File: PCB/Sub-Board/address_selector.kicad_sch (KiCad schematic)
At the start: 10 parts, among them SW1 SW_DIP_x07

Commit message: Sub Board PCB: PCB Layout (wip)
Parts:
- R10, R11, R12, R13, R5, R6, R7, R8, R9: footprint Resistor_SMD:R_0603_1608Metric -> Resistor_SMD:R_0402_1005Metric
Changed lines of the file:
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@@
 			)
 		)
-		(property "Footprint" "Resistor_SMD:R_0603_1608Metric"
+		(property "Footprint" "Resistor_SMD:R_0402_1005Metric"
 			(at 87.122 83.82 90)
 			(effects
@@
 			)
 		)
-		(property "Footprint" "Resistor_SMD:R_0603_1608Metric"
+		(property "Footprint" "Resistor_SMD:R_0402_1005Metric"
 			(at 109.982 83.82 90)
 			(effects
@@
 			)
 		)
-		(property "Footprint" "Resistor_SMD:R_0603_1608Metric"
+		(property "Footprint" "Resistor_SMD:R_0402_1005Metric"
 			(at 79.502 83.82 90)
 			(effects
@@
 			)
 		)
-		(property "Footprint" "Resistor_SMD:R_0603_1608Metric"
+		(property "Footprint" "Resistor_SMD:R_0402_1005Metric"
 			(at 117.602 55.88 90)
 			(effects
@@
 			)
 		)
-		(property "Footprint" "Resistor_SMD:R_0603_1608Metric"
+		(property "Footprint" "Resistor_SMD:R_0402_1005Metric"
 			(at 94.742 83.82 90)
 			(effects
@@
 			)
 		)
-		(property "Footprint" "Resistor_SMD:R_0603_1608Metric"
+		(property "Footprint" "Resistor_SMD:R_0402_1005Metric"
 			(at 64.262 83.82 90)
 			(effects
@@
 			)
 		)
-		(property "Footprint" "Resistor_SMD:R_0603_1608Metric"
+		(property "Footprint" "Resistor_SMD:R_0402_1005Metric"
 			(at 39.37 71.628 90)
 			(effects
@@
 			)
 		)
-		(property "Footprint" "Resistor_SMD:R_0603_1608Metric"
+		(property "Footprint" "Resistor_SMD:R_0402_1005Metric"
 			(at 102.362 83.82 90)
 			(effects
@@
 			)
 		)
-		(property "Footprint" "Resistor_SMD:R_0603_1608Metric"
+		(property "Footprint" "Resistor_SMD:R_0402_1005Metric"
 			(at 71.882 83.82 90)
 			(effects

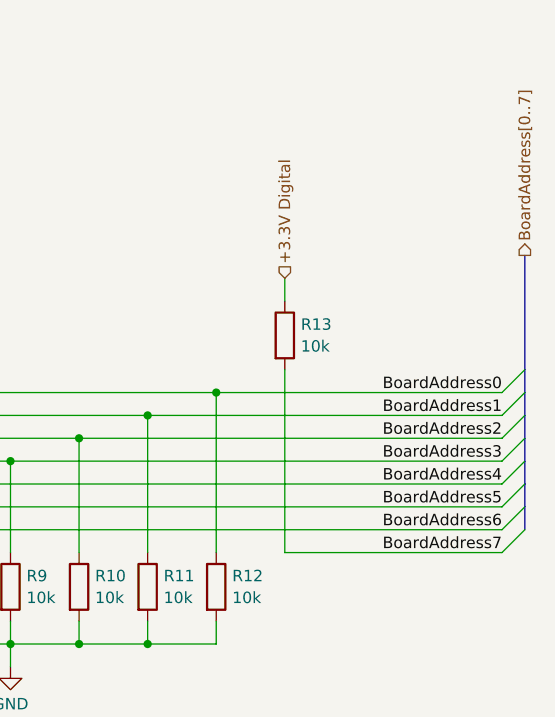
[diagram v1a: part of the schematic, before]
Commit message: Sub Board PCB: Parts Placement (wip)
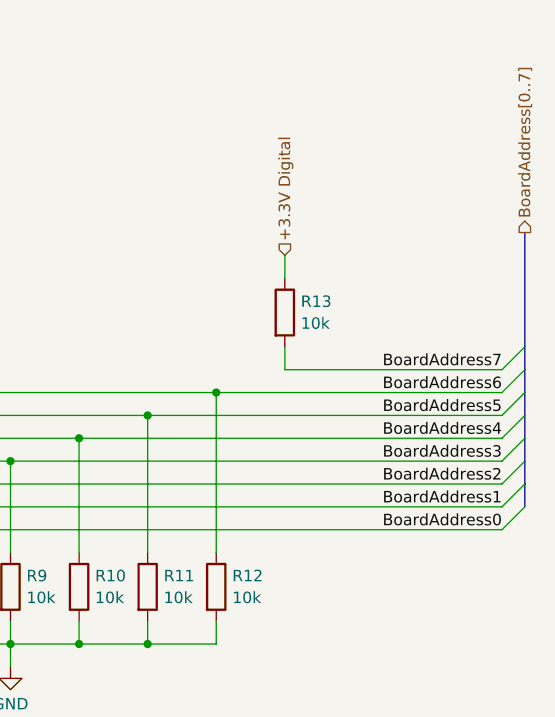
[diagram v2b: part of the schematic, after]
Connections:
- net BoardAddress0: now also R6.1, SW1.8; no longer R12.1, SW1.14
- net BoardAddress1: now also R7.1, SW1.9; no longer R11.1, SW1.13
- net BoardAddress2: now also R8.1, SW1.10; no longer R10.1, SW1.12
- net BoardAddress4: now also R10.1, SW1.12; no longer R8.1, SW1.10
- net BoardAddress5: now also R11.1, SW1.13; no longer R7.1, SW1.9
- net BoardAddress6: now also R12.1, SW1.14; no longer R6.1, SW1.8
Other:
- moved on the sheet: R13
